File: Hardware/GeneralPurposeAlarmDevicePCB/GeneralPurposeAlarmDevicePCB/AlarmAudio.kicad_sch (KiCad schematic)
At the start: 13 parts, among them J601 22-23-2021, Q601 MMBT2222A-7-F, Q602 MMBT2907ALT1G

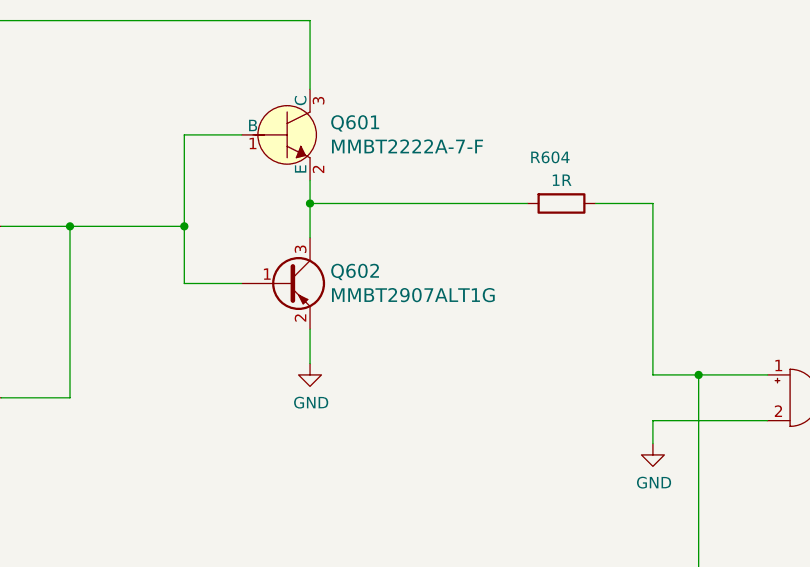
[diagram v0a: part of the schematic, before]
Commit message: Fix incorrect Q602 emiter collector orientation.
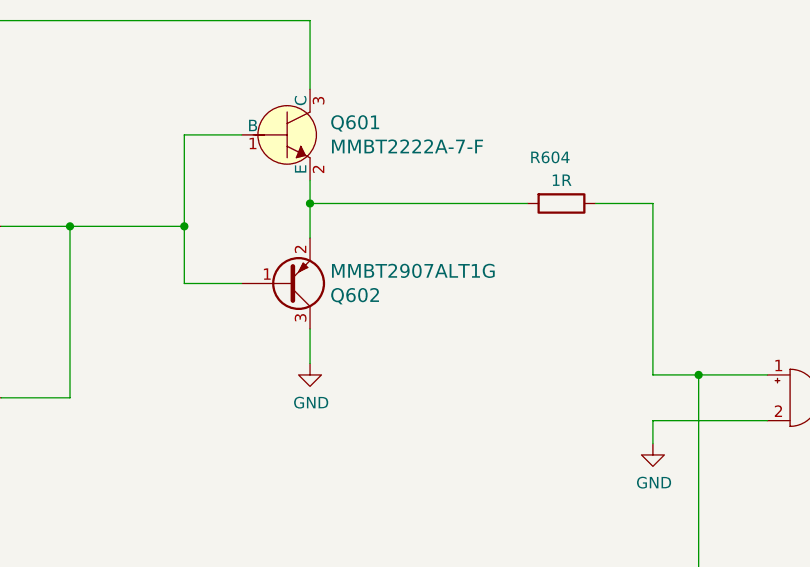
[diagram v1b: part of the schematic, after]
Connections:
- net GND: now also Q602.3 (C); no longer Q602.2 (E)
- net at Q601.2 (E), R604.2: now also Q602.2 (E); no longer Q602.3 (C)
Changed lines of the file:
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@@
     (pin "2")
   )
-  (symbol (lib_id "Device:Q_PNP_BEC") (at 134.62 77.47 0) (unit 1)
+  (symbol (lib_id "Device:Q_PNP_BEC") (at 134.62 77.47 0) (mirror x) (unit 1)
     (in_bom yes) (on_board yes)
-    (property "Reference" "Q602" (id 0) (at 139.3952 76.1238 0)
+    (property "Reference" "Q602" (id 0) (at 139.3952 78.8162 0)
       (effects (font (size 1.524 1.524)) (justify left))
     )
-    (property "Value" "MMBT2907ALT1G" (id 1) (at 139.3952 78.8162 0)
+    (property "Value" "MMBT2907ALT1G" (id 1) (at 139.3952 76.1238 0)
       (effects (font (size 1.524 1.524)) (justify left))
     )
-    (property "Footprint" "digikey-footprints:SOT-23-3" (id 2) (at 139.7 74.93 0)
+    (property "Footprint" "digikey-footprints:SOT-23-3" (id 2) (at 139.7 80.01 0)
       (effects (font (size 1.27 1.27)) hide)
     )
@@
       (effects (font (size 1.27 1.27)) hide)
     )
-    (property "Digi-Key_PN" "MMBT2907ALT1GOSCT-ND" (id 4) (at 139.7 67.31 0)
+    (property "Digi-Key_PN" "MMBT2907ALT1GOSCT-ND" (id 4) (at 139.7 87.63 0)
       (effects (font (size 1.524 1.524)) (justify left) hide)
     )
-    (property "MPN" "MMBT2907ALT1G" (id 5) (at 139.7 64.77 0)
+    (property "MPN" "MMBT2907ALT1G" (id 5) (at 139.7 90.17 0)
       (effects (font (size 1.524 1.524)) (justify left) hide)
     )
-    (property "Category" "Discrete Semiconductor Products" (id 6) (at 139.7 62.23 0)
+    (property "Category" "Discrete Semiconductor Products" (id 6) (at 139.7 92.71 0)
       (effects (font (size 1.524 1.524)) (justify left) hide)
     )
-    (property "Family" "Transistors - Bipolar (BJT) - Single" (id 7) (at 139.7 59.69 0)
+    (property "Family" "Transistors - Bipolar (BJT) - Single" (id 7) (at 139.7 95.25 0)
       (effects (font (size 1.524 1.524)) (justify left) hide)
     )
-    (property "DK_Datasheet_Link" "http://www.onsemi.com/pub/Collateral/MMBT2907ALT1-D.PDF" (id 8) (at 139.7 57.15 0)
+    (property "DK_Datasheet_Link" "http://www.onsemi.com/pub/Collateral/MMBT2907ALT1-D.PDF" (id 8) (at 139.7 97.79 0)
       (effects (font (size 1.524 1.524)) (justify left) hide)
     )
-    (property "DK_Detail_Page" "/product-detail/en/on-semiconductor/MMBT2907ALT1G/MMBT2907ALT1GOSCT-ND/1139812" (id 9) (at 139.7 54.61 0)
+    (property "DK_Detail_Page" "/product-detail/en/on-semiconductor/MMBT2907ALT1G/MMBT2907ALT1GOSCT-ND/1139812" (id 9) (at 139.7 100.33 0)
       (effects (font (size 1.524 1.524)) (justify left) hide)
     )
-    (property "Description" "TRANS PNP 60V 0.6A SOT23" (id 10) (at 139.7 52.07 0)
+    (property "Description" "TRANS PNP 60V 0.6A SOT23" (id 10) (at 139.7 102.87 0)
       (effects (font (size 1.524 1.524)) (justify left) hide)
     )
-    (property "Manufacturer" "ON Semiconductor" (id 11) (at 139.7 49.53 0)
+    (property "Manufacturer" "ON Semiconductor" (id 11) (at 139.7 105.41 0)
       (effects (font (size 1.524 1.524)) (justify left) hide)
     )
-    (property "Status" "Active" (id 12) (at 139.7 46.99 0)
+    (property "Status" "Active" (id 12) (at 139.7 107.95 0)
       (effects (font (size 1.524 1.524)) (justify left) hide)
     )
